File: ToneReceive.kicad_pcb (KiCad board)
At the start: 2 copper layers, 175.3 x 96.5 mm, 83 parts, among them J1 XLR3, J10 1/4" Jack, J11 1/4" Jack, J12 1/4" Jack, J13 1/4" Jack, J14 9v DC in, J2 1/4" Jack, J3 1/4" Jack, J4 1/4" Jack, J5 1/4" Jack, J6 1/4" Jack, J7 1/4" Jack, J8 1/4" Jack, J9 1/4" Jack, K1 G6K-2, K2 G6K-2, K3 G6K-2, K4 G6K-2, K5 G6K-2, K6 G6K-2, Q1 PN2222A, Q10 PN2222A, Q11 PN2222A, Q12 PN2222A, Q2 PN2222A, Q3 PN2222A, Q4 PN2222A, Q5 PN2222A, Q6 PN2222A, Q7 PN2222A, Q8 PN2222A, Q9 PN2222A, SW1 SW_DPDT_x2, SW2 SW_DPDT_x2, SW3 SW_DPDT_x2, SW4 SW_DPDT_x2, SW5 SW_DPDT_x2, SW6 SW_DPDT_x2, U1 MT8870DE, U2 74HC238, U3 VX7805-500, Y1 3.579545 .1%

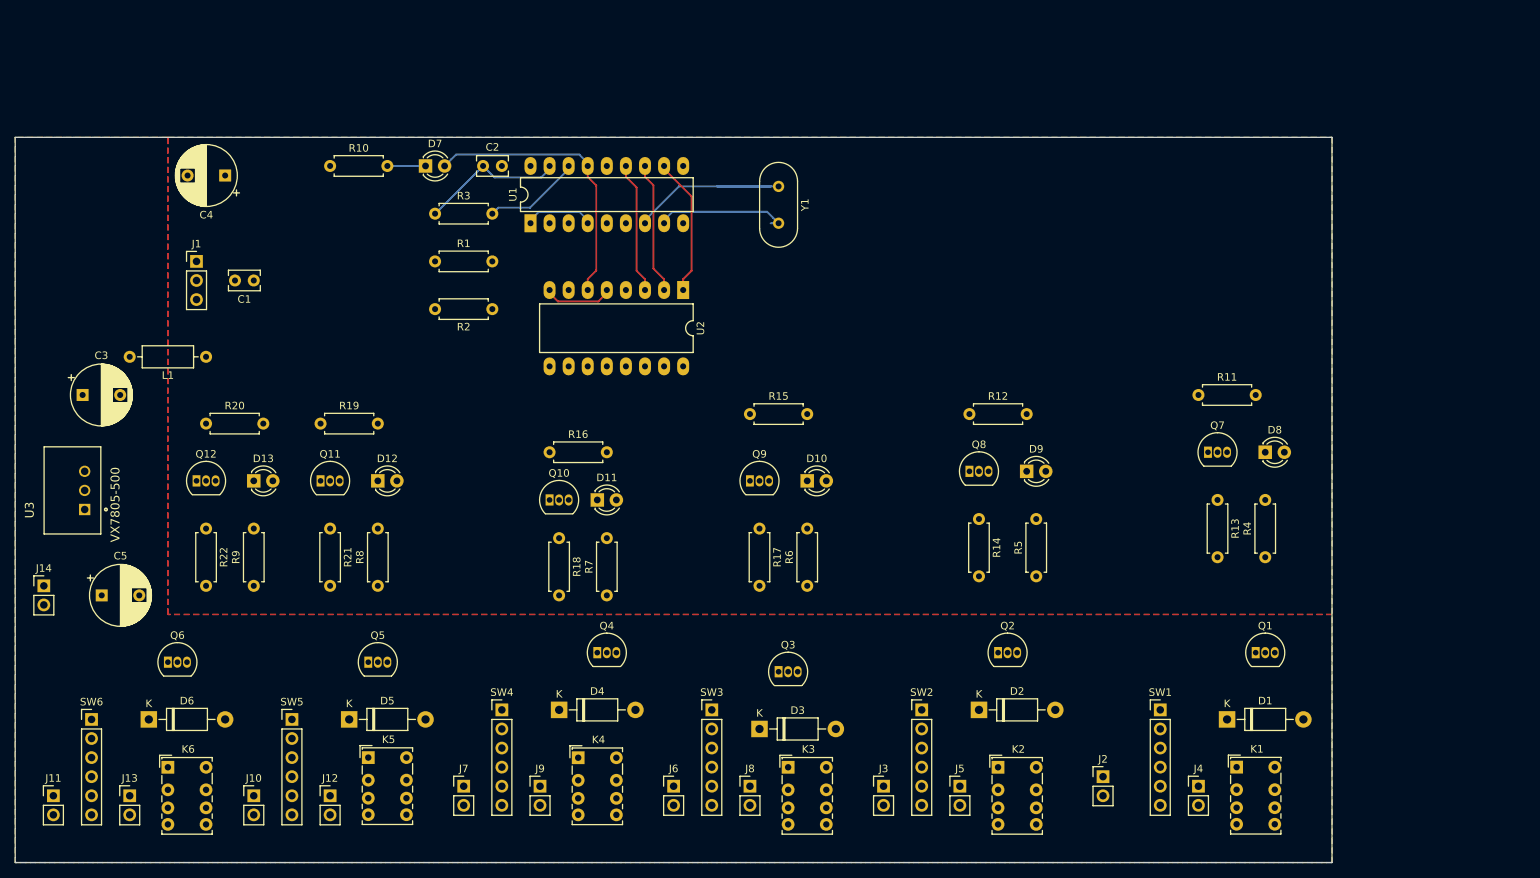
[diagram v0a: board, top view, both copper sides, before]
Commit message: layout PCB
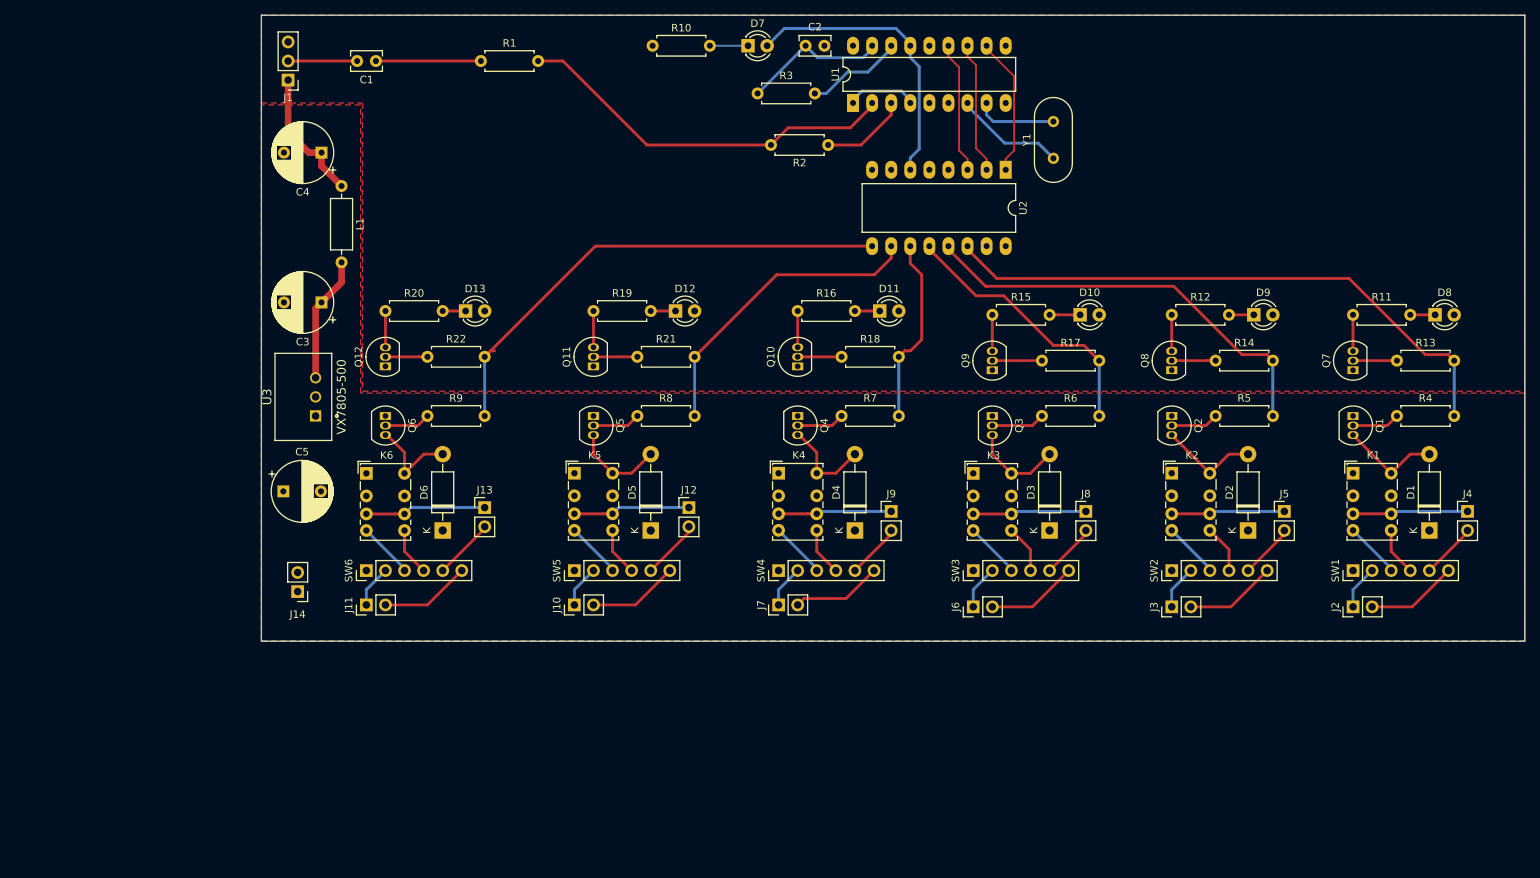
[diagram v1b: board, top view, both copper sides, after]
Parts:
- moved J12 61.2 mm to (117.6, 117.9)
- moved J13 60.9 mm to (90.4, 117.9)
- moved J9 59.3 mm to (144.5, 118.4)
- moved J8 57.8 mm to (170.4, 118.4)
- moved J5 56.6 mm to (196.8, 118.4)
- moved J4 51.2 mm to (221.2, 118.4)
- moved R2 49.8 mm to (136.1, 69.6)
- moved J10 49.7 mm to (102.4, 130.8), turned to 90 degrees
- moved J11 48.8 mm to (74.7, 130.8), turned to 90 degrees
- moved J7 48.4 mm to (129.5, 130.8), turned to 90 degrees
- moved D5 47.4 mm to (112.5, 120.9), turned to 90 degrees
- moved K6 47.2 mm to (74.7, 113.3)
- moved R21 46.8 mm to (110.7, 97.8), turned to 0 degrees
- moved D3 46.8 mm to (165.6, 120.9), turned to 90 degrees
- moved K5 46.7 mm to (102.4, 113.3)
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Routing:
- net BTN1: track 0.00 -> 78.7 mm
- net BTN6: track 0.00 -> 67.2 mm
- net BTN2: track 0.00 -> 57.1 mm
- net Net-(R1-Pad2): track 0.00 -> 51.6 mm
- net BTN5: track 0.00 -> 41.1 mm
- net BTN3: track 0.00 -> 36.5 mm
- net BTN4: track 0.00 -> 24.9 mm
- net +5V: track 0.00 -> 18.0 mm
- net Net-(C3-Pad1): track 0.00 -> 16.8 mm
- net Net-(J13-Pad1): track 0.00 -> 16.1 mm
- net Net-(J12-Pad1): track 0.00 -> 15.6 mm
- net Net-(J4-Pad1): track 0.00 -> 15.4 mm
- net Net-(J8-Pad1): track 0.00 -> 15.1 mm
- net Net-(J9-Pad1): track 0.00 -> 15.1 mm
- net Net-(J5-Pad1): track 0.00 -> 15.1 mm
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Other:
- board size 175.3 x 96.5 mm -> 168.1 x 83.3 mm

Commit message: PCB Layout
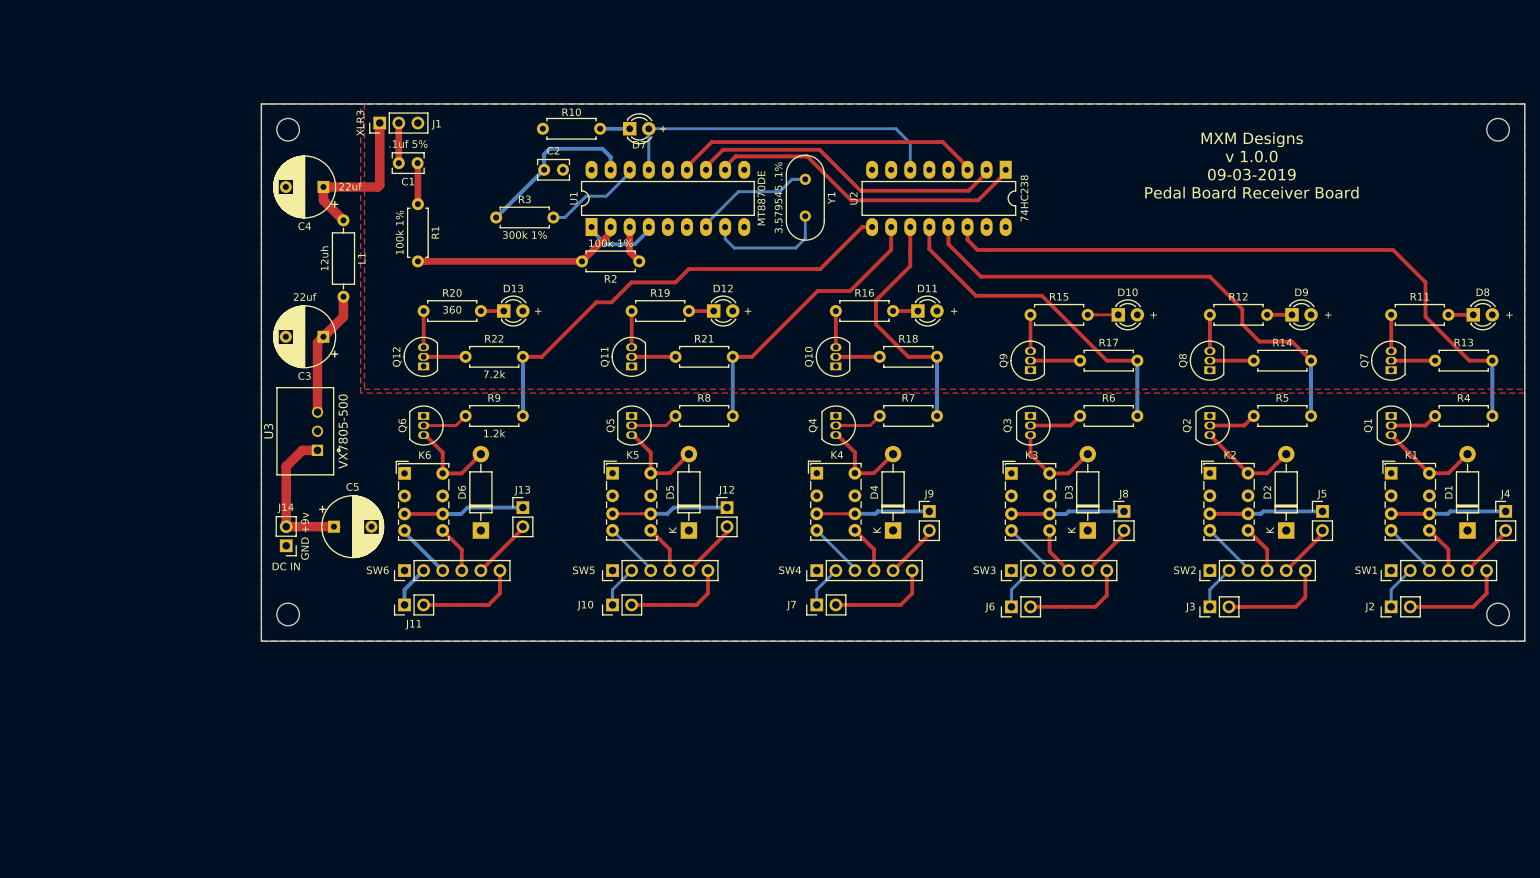
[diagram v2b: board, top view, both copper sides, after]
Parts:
- added H1: MountingHole, MountingHole:MountingHole_3mm, F.Cu at (64.3, 67.6)
- added H2: MountingHole, MountingHole:MountingHole_3mm, F.Cu at (64.3, 132.1)
- added H3: MountingHole, MountingHole:MountingHole_3mm, F.Cu at (225.3, 67.6)
- added H4: MountingHole, MountingHole:MountingHole_3mm, F.Cu at (225.3, 132.1)
- C1: value 100nf 5% -> .1uf 5%
- U2: footprint Package_DIP:DIP-16_W10.16mm_LongPads -> Package_DIP:DIP-16_W7.62mm_LongPads
- moved R3 38.5 mm to (91.9, 79.2)
- moved U1 38.5 mm to (104.6, 80.5)
- moved C2 38.5 mm to (98.3, 72.9)
- moved Y1 33.1 mm to (133.1, 74.2), turned to 270 degrees
- moved R2 29.5 mm to (111.0, 85.1)
- moved R1 20.8 mm to (81.5, 77.5), turned to 270 degrees
- moved D7 19.2 mm to (109.7, 67.4)
- moved R10 18.3 mm to (98.2, 67.4)
- moved C1 14.7 mm to (81.5, 72.0)
- moved J1 13.5 mm to (76.5, 66.7), turned to 90 degrees
- moved C5 8.21 mm to (70.4, 120.4)
- moved J14 6.28 mm to (64.0, 122.9)
- moved D1 5.08 mm to (221.2, 120.9)
- moved D10 5.08 mm to (174.8, 92.2)
- moved D2 5.08 mm to (197.1, 120.9)
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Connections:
- K1 pad 2: (no net) -> Net-(K1-Pad2)
- K1 pad 7: (no net) -> Net-(K1-Pad7)
- K2 pad 2: (no net) -> Net-(K2-Pad2)
- K2 pad 7: (no net) -> Net-(K2-Pad7)
- K3 pad 2: (no net) -> Net-(K3-Pad2)
- K3 pad 7: (no net) -> Net-(K3-Pad7)
- K4 pad 2: (no net) -> Net-(K4-Pad2)
- K4 pad 7: (no net) -> Net-(K4-Pad7)
- K5 pad 2: (no net) -> Net-(K5-Pad2)
- K5 pad 7: (no net) -> Net-(K5-Pad7)
- K6 pad 2: (no net) -> Net-(K6-Pad2)
- K6 pad 7: (no net) -> Net-(K6-Pad7)
- SW1 pad 1: (no net) -> Net-(SW1-Pad1)
- SW2 pad 1: (no net) -> Net-(SW2-Pad1)
- SW3 pad 1: (no net) -> Net-(SW3-Pad1)
- SW4 pad 1: (no net) -> Net-(SW4-Pad1)
- SW5 pad 1: (no net) -> Net-(SW5-Pad1)
- SW6 pad 1: (no net) -> Net-(SW6-Pad1)
- U1 pad 14: (no net) -> Net-(U1-Pad14)
- U1 pad 6: (no net) -> Net-(U1-Pad6)
- U2 pad 15: (no net) -> Net-(U2-Pad15)
- U2 pad 7: (no net) -> Net-(U2-Pad7)
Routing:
- net A0: track 18.5 -> 52.6 mm
- net A1: track 17.6 -> 42.3 mm
- net A2: track 17.6 -> 40.9 mm
- net Net-(R1-Pad2): track 51.6 -> 28.4 mm
- net +9V: track 0.00 -> 19.7 mm
- net BTN4: track 24.9 -> 42.1 mm
- net BTN1: track 78.7 -> 88.3 mm
- net Net-(C1-Pad1): track 14.0 -> 5.48 mm
- net BTN2: track 57.1 -> 65.5 mm
- net BTN3: track 36.5 -> 44.1 mm
- net Net-(D7-Pad2): track 38.7 -> 45.8 mm
- net Net-(R2-Pad1): track 11.6 -> 5.10 mm
- net Net-(U1-Pad8): track 10.8 -> 16.7 mm
- net BTN6: track 67.2 -> 61.5 mm
- net Net-(C1-Pad2): track 9.18 -> 5.33 mm
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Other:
- board size 168.1 x 83.3 mm -> 168.1 x 71.5 mm
- board text added: "+"
- board text added: "+9v"
- board text added: "DC IN"
- board text added: "GND"
- board text added: "MXM Designs v 1.0.0 09-03-2019 Pedal Board Receiver Board"
